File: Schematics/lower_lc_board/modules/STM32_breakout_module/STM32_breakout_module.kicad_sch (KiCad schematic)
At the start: 43 parts, among them J2 SWD_CONN, J3 USB_C_CONN, SW1 SW_STM_RESET, SW2 SW_STM_BOOT_MODE, U5 STM32F103CBT6, U6 W25Q128JVS, U7 ISO1044BDR, U8 CP2102N-Axx-xQFN28, Y1 X322516MMB4SI

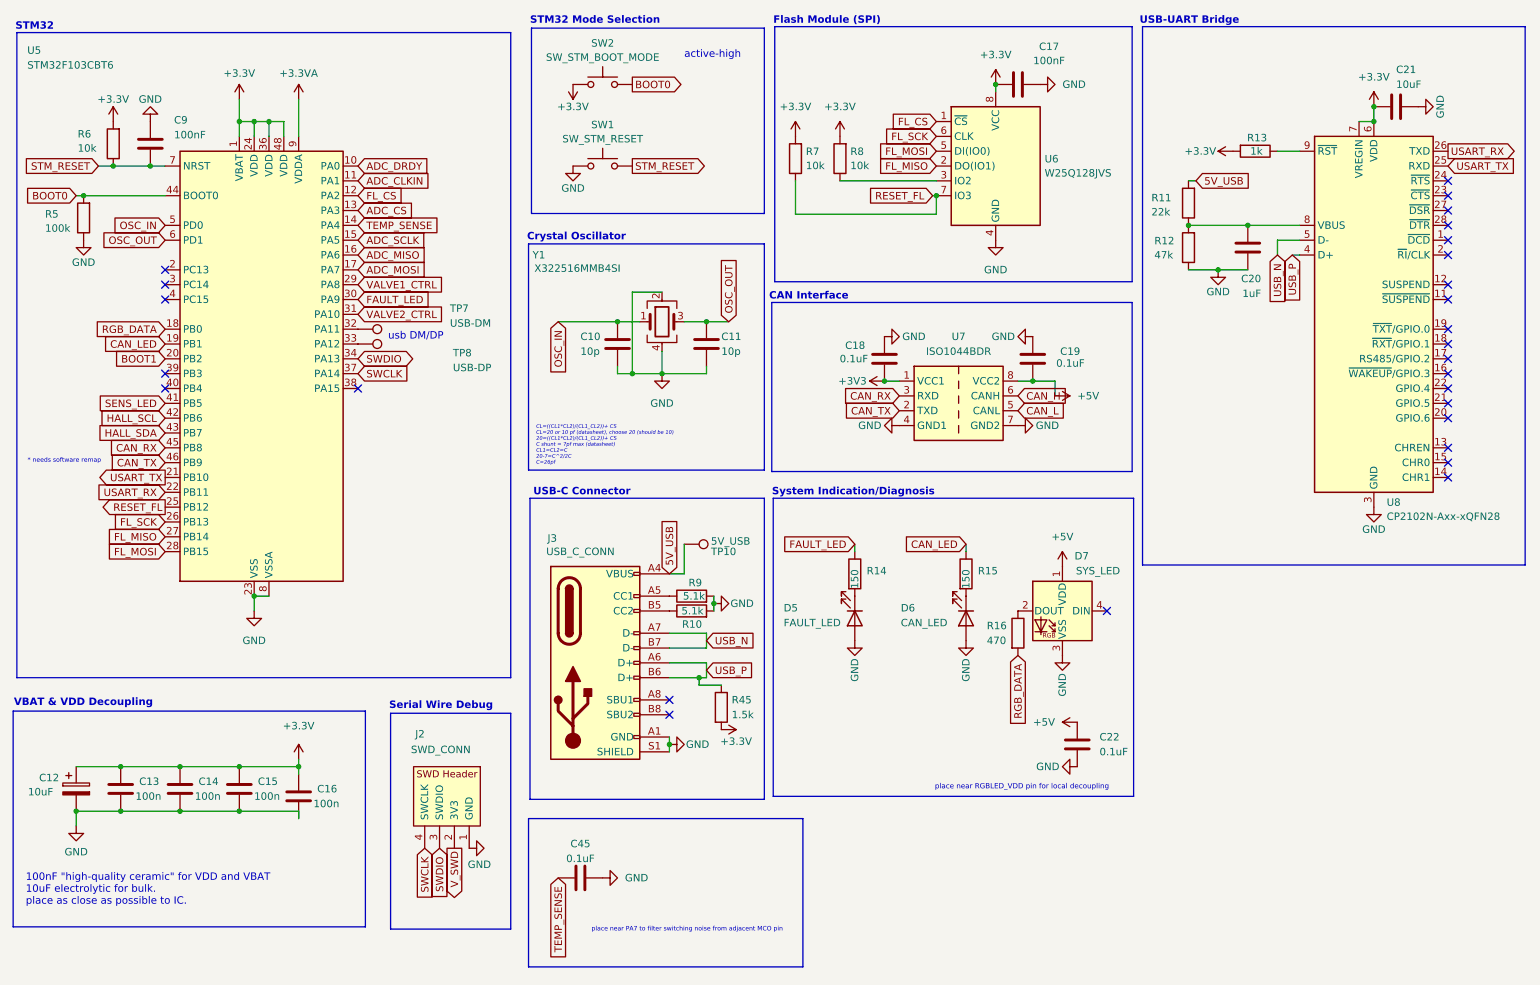
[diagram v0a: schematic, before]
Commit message: more layout work, add testing code
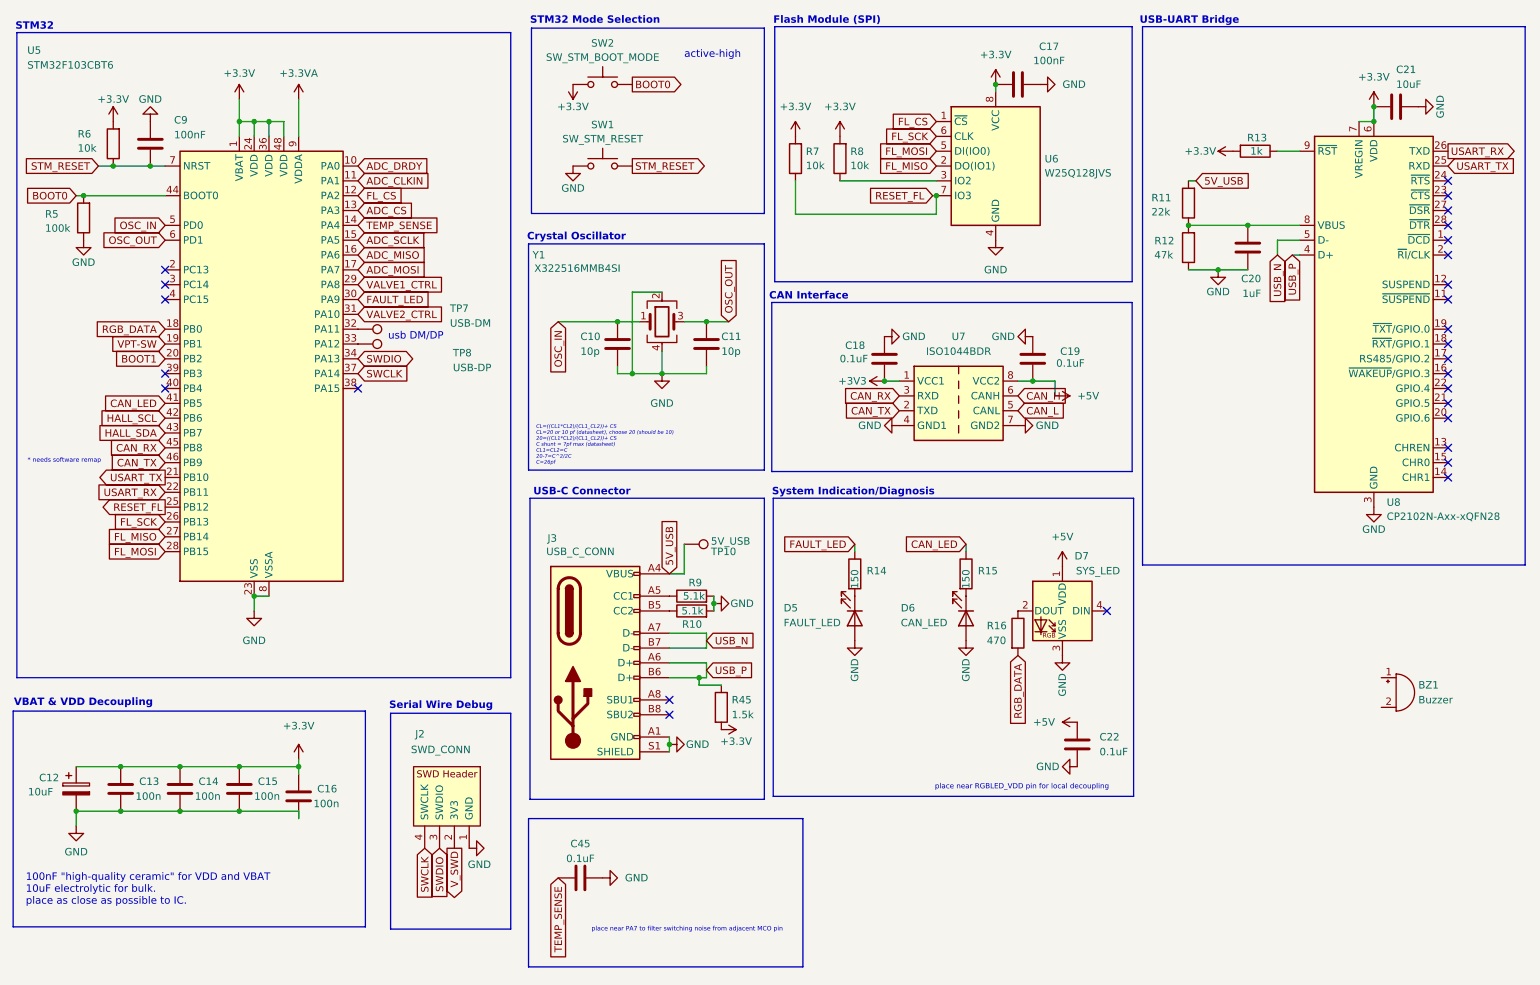
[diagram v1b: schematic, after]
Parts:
- added BZ1: Buzzer, symbol Device:Buzzer
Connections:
- net SENS_LED is gone; now on net CAN_LED: U5.41 (PB5)
- net CAN_LED: no longer U5.19 (PB1)
- new net VPT-SW: U5.19 (PB1)
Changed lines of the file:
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@@
 		)
 	)
-	(global_label "CAN_LED"
+	(global_label "FL_MISO"
 		(shape input)
-		(at 41.91 78.74 180)
+		(at 173.99 48.26 180)
 		(fields_autoplaced yes)
 		(effects
@@
 		)
 		(property "Intersheetrefs" "${INTERSHEET_REFS}"
-			(at 30.821 78.74 0)
+			(at 163.3243 48.26 0)
 			(effects
 				(font
@@
 		)
 	)
-	(global_label "FL_MISO"
+	(global_label "CAN_H"
 		(shape input)
-		(at 173.99 48.26 180)
+		(at 187.96 87.63 0)
 		(fields_autoplaced yes)
 		(effects
@@
 				(size 1.27 1.27)
 			)
-			(justify right)
+			(justify left)
 		)
 		(property "Intersheetrefs" "${INTERSHEET_REFS}"
-			(at 163.3243 48.26 0)
+			(at 196.9324 87.63 0)
 			(effects
 				(font
 					(size 1.27 1.27)
 				)
-				(justify right)
+				(justify left)
 				(hide yes)
 			)
 		)
 	)
-	(global_label "CAN_H"
+	(global_label "CAN_RX"
 		(shape input)
-		(at 187.96 87.63 0)
+		(at 167.64 87.63 180)
 		(fields_autoplaced yes)
 		(effects
@@
 				(size 1.27 1.27)
 			)
-			(justify left)
+			(justify right)
 		)
 		(property "Intersheetrefs" "${INTERSHEET_REFS}"
-			(at 196.9324 87.63 0)
+			(at 157.5186 87.63 0)
 			(effects
 				(font
 					(size 1.27 1.27)
 				)
-				(justify left)
+				(justify right)
 				(hide yes)
 			)
 		)
 	)
-	(global_label "CAN_RX"
+	(global_label "VPT-SW"
 		(shape input)
-		(at 167.64 87.63 180)
+		(at 41.91 78.74 180)
 		(fields_autoplaced yes)
 		(effects
@@
 		)
 		(property "Intersheetrefs" "${INTERSHEET_REFS}"
-			(at 157.5186 87.63 0)
+			(at 31.3653 78.74 0)
 			(effects
 				(font
@@
 		)
 	)
-	(global_label "ADC_MOSI"
+	(global_label "CAN_LED"
 		(shape input)
-		(at 74.93 66.04 0)
+		(at 41.91 88.9 180)
 		(fields_autoplaced yes)
 		(effects
@@
 				(size 1.27 1.27)
 			)
-			(justify left)
+			(justify right)
 		)
 		(property "Intersheetrefs" "${INTERSHEET_REFS}"
-			(at 87.1076 66.04 0)
+			(at 30.821 88.9 0)
 			(effects
 				(font
 					(size 1.27 1.27)
 				)
-				(justify left)
+				(justify right)
 				(hide yes)
 			)
 		)
 	)
-	(global_label "FL_MISO"
+	(global_label "ADC_MOSI"
 		(shape input)
-		(at 41.91 111.76 180)
+		(at 74.93 66.04 0)
 		(fields_autoplaced yes)
 		(effects
@@
 				(size 1.27 1.27)
 			)
-			(justify right)
+			(justify left)
 		)
 		(property "Intersheetrefs" "${INTERSHEET_REFS}"
-			(at 31.2443 111.76 0)
+			(at 87.1076 66.04 0)
 			(effects
 				(font
 					(size 1.27 1.27)
 				)
-				(justify right)
+				(justify left)
 				(hide yes)
 			)
 		)
 	)
-	(global_label "RESET_FL"
-		(shape output)
-		(at 41.91 106.68 180)
+	(global_label "FL_MISO"
+		(shape input)
+		(at 41.91 111.76 180)
 		(fields_autoplaced yes)
 		(effects
@@
 		)
 		(property "Intersheetrefs" "${INTERSHEET_REFS}"
-			(at 30.0954 106.68 0)
+			(at 31.2443 111.76 0)
 			(effects
 				(font
@@
 		)
 	)
-	(global_label "SENS_LED"
-		(shape input)
-		(at 41.91 88.9 180)
+	(global_label "RESET_FL"
+		(shape output)
+		(at 41.91 106.68 180)
 		(fields_autoplaced yes)
 		(effects
@@
 		)
 		(property "Intersheetrefs" "${INTERSHEET_REFS}"
-			(at 29.6116 88.9 0)
+			(at 30.0954 106.68 0)
 			(effects
 				(font
@@
 					(unit 1)
 				)
+			)
+		)
+	)
+	(symbol
+		(lib_id "Device:Buzzer")
+		(at 252.73 138.43 0)
+		(unit 1)
+		(exclude_from_sim no)
+		(in_bom yes)
+		(on_board yes)
+		(dnp no)
+		(fields_autoplaced yes)
+		(property "Reference" "BZ1"
+			(at 256.54 137.1599 0)
+			(effects
+				(font
+					(size 1.27 1.27)
+				)
+				(justify left)
+			)
+		)
+		(property "Value" "Buzzer"
+			(at 256.54 139.6999 0)
+			(effects
+				(font
+					(size 1.27 1.27)
+				)
+				(justify left)
+			)
+		)
+		(property "Footprint" ""
+			(at 252.095 135.89 90)
+			(effects
+				(font
+					(size 1.27 1.27)
+				)
+				(hide yes)
+			)
+		)
+		(property "Datasheet" "~"
+			(at 252.095 135.89 90)
+			(effects
+				(font
+					(size 1.27 1.27)
+				)
+				(hide yes)
+			)
+		)
+		(property "Description" "Buzzer, polarized"
+			(at 252.73 138.43 0)
+			(effects
+				(font
+					(size 1.27 1.27)
+				)
+				(hide yes)
+			)
+		)
+		(pin "1"
+		)
+		(pin "2"
+		)
+		(instances
+			(project ""
+				(path "/d63798c4-e363-437e-9012-e4aff32e6642/925ef91a-c900-4b94-a159-606c279d7192"
+					(reference "BZ1")
+					(unit 1)
+				)
